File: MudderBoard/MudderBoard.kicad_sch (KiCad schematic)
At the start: 0 parts

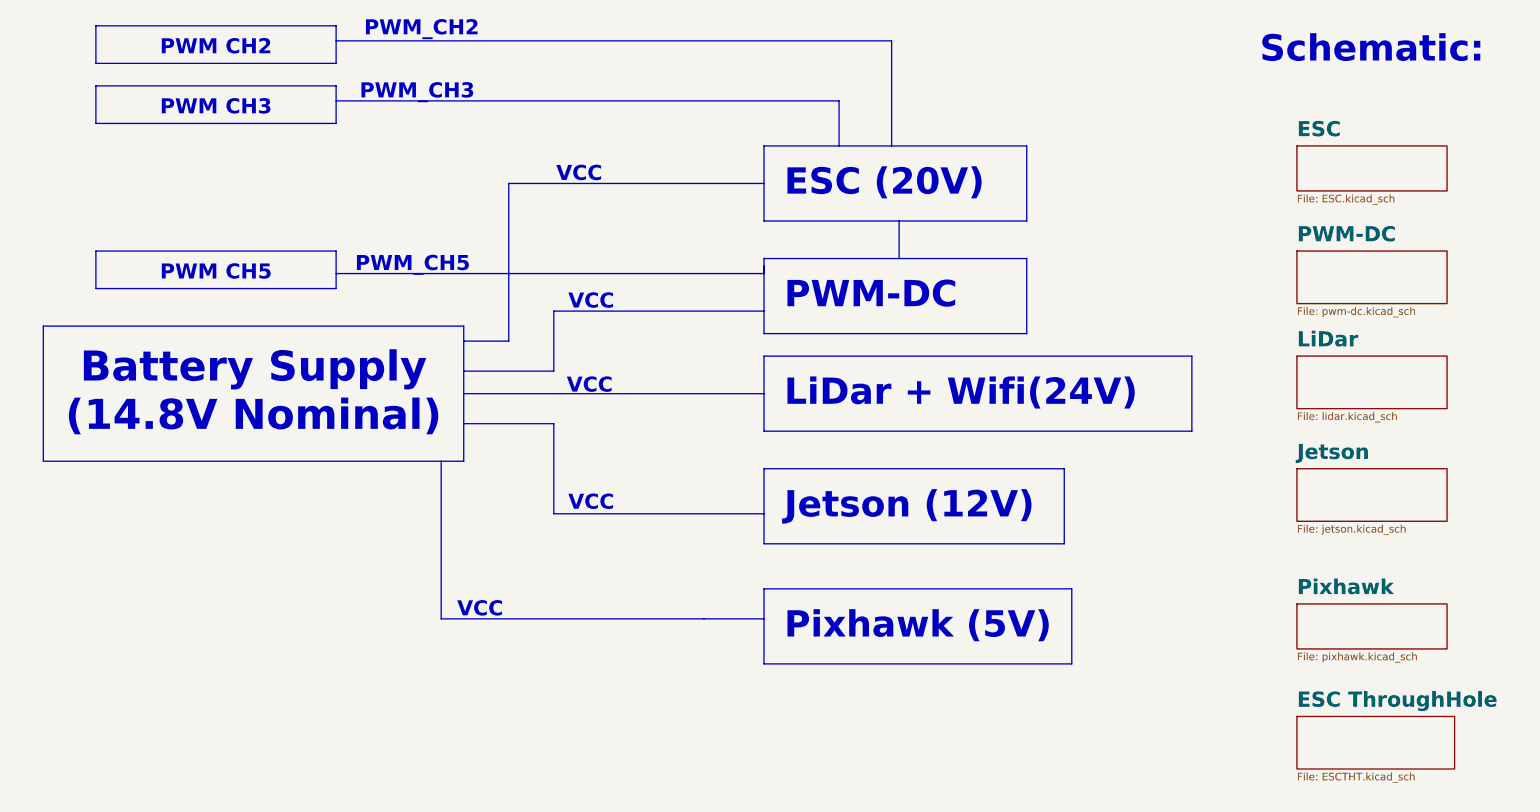
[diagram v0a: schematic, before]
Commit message: added jetson circuit
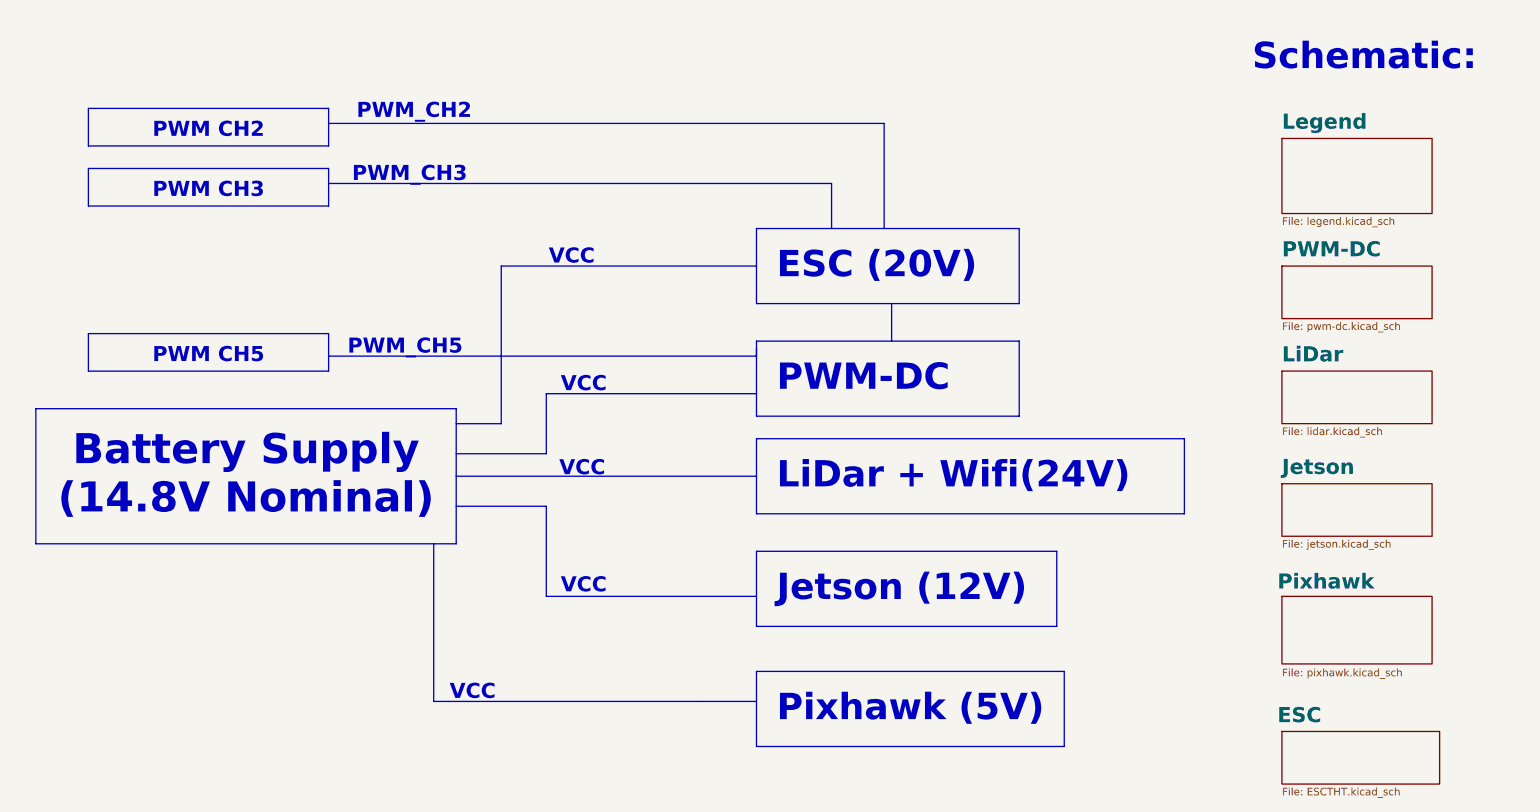
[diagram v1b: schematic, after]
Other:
- removed sheet ESC ThroughHole
- added sheet Legend (legend.kicad_sch)
- sheet ESC: file ESC.kicad_sch -> ESCTHT.kicad_sch
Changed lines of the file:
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@@
 	(polyline
 		(pts
-			(xy 93.98 74.93) (xy 109.22 74.93)
+			(xy 92.71 88.9) (xy 107.95 88.9)
 		)
 		(stroke
@@
 	(polyline
 		(pts
-			(xy 72.39 58.42) (xy 144.78 58.42)
+			(xy 71.12 72.39) (xy 143.51 72.39)
 		)
 		(stroke
@@
 	(polyline
 		(pts
-			(xy 167.64 49.53) (xy 167.64 55.88)
+			(xy 166.37 63.5) (xy 166.37 69.85)
 		)
 		(stroke
@@
 	(polyline
 		(pts
-			(xy 72.39 29.21) (xy 157.48 29.21)
+			(xy 71.12 43.18) (xy 156.21 43.18)
 		)
 		(stroke
@@
 	(polyline
 		(pts
-			(xy 101.6 69.85) (xy 101.6 43.18)
+			(xy 100.33 83.82) (xy 100.33 57.15)
 		)
 		(stroke
@@
 	(polyline
 		(pts
-			(xy 109.22 74.93) (xy 109.22 64.77)
+			(xy 107.95 88.9) (xy 107.95 78.74)
 		)
 		(stroke
@@
 	(polyline
 		(pts
-			(xy 109.22 64.77) (xy 144.78 64.77)
+			(xy 107.95 78.74) (xy 143.51 78.74)
 		)
 		(stroke
@@
 	(polyline
 		(pts
-			(xy 157.48 29.21) (xy 157.48 36.83)
+			(xy 156.21 43.18) (xy 156.21 50.8)
 		)
 		(stroke
@@
 	(polyline
 		(pts
-			(xy 144.78 57.15) (xy 144.78 58.42)
+			(xy 143.51 71.12) (xy 143.51 72.39)
 		)
 		(stroke
@@
 	(polyline
 		(pts
-			(xy 90.17 90.17) (xy 90.17 116.84)
+			(xy 88.9 104.14) (xy 88.9 130.81)
 		)
 		(stroke
@@
 	(polyline
 		(pts
-			(xy 93.98 78.74) (xy 144.78 78.74)
+			(xy 92.71 92.71) (xy 143.51 92.71)
 		)
 		(stroke
@@
 	(polyline
 		(pts
-			(xy 134.62 116.84) (xy 144.78 116.84)
+			(xy 133.35 130.81) (xy 143.51 130.81)
 		)
 		(stroke
@@
 	(polyline
 		(pts
-			(xy 90.17 116.84) (xy 134.62 116.84)
+			(xy 88.9 130.81) (xy 133.35 130.81)
 		)
 		(stroke
@@
 	(polyline
 		(pts
-			(xy 166.37 19.05) (xy 166.37 36.83)
+			(xy 165.1 33.02) (xy 165.1 50.8)
 		)
 		(stroke
@@
 	(polyline
 		(pts
-			(xy 72.39 19.05) (xy 166.37 19.05)
+			(xy 71.12 33.02) (xy 165.1 33.02)
 		)
 		(stroke
@@
 	(polyline
 		(pts
-			(xy 144.78 99.06) (xy 109.22 99.06)
+			(xy 143.51 113.03) (xy 107.95 113.03)
 		)
 		(stroke
@@
 	(polyline
 		(pts
-			(xy 109.22 99.06) (xy 109.22 83.82)
+			(xy 107.95 113.03) (xy 107.95 97.79)
 		)
 		(stroke
@@
 	(polyline
 		(pts
-			(xy 93.98 69.85) (xy 101.6 69.85)
+			(xy 92.71 83.82) (xy 100.33 83.82)
 		)
 		(stroke
@@
 	(polyline
 		(pts
-			(xy 101.6 43.18) (xy 144.78 43.18)
+			(xy 100.33 57.15) (xy 143.51 57.15)
 		)
 		(stroke
@@
 	(polyline
 		(pts
-			(xy 93.98 83.82) (xy 109.22 83.82)
+			(xy 92.71 97.79) (xy 107.95 97.79)
 		)
 		(stroke
@@
 	(text_box "PWM CH2"
 		(exclude_from_sim no)
-		(at 31.75 16.51 0)
+		(at 30.48 30.48 0)
 		(size 40.64 6.35)
 		(stroke
@@
 	(text_box "PWM CH5"
 		(exclude_from_sim no)
-		(at 31.75 54.61 0)
+		(at 30.48 68.58 0)
 		(size 40.64 6.35)
 		(stroke
@@
 	(text_box "Pixhawk (5V)"
 		(exclude_from_sim no)
-		(at 144.78 111.76 0)
+		(at 143.51 125.73 0)
 		(size 52.07 12.7)
 		(stroke
@@
 	(text_box "Jetson (12V)"
 		(exclude_from_sim no)
-		(at 144.78 91.44 0)
+		(at 143.51 105.41 0)
 		(size 50.8 12.7)
 		(stroke
@@
 	(text_box "LiDar + Wifi(24V)"
 		(exclude_from_sim no)
-		(at 144.78 72.39 0)
+		(at 143.51 86.36 0)
 		(size 72.39 12.7)
 		(stroke
@@
 	(text_box "PWM-DC"
 		(exclude_from_sim no)
-		(at 144.78 55.88 0)
+		(at 143.51 69.85 0)
 		(size 44.45 12.7)
 		(stroke
@@
 	(text_box "ESC (20V)"
 		(exclude_from_sim no)
-		(at 144.78 36.83 0)
+		(at 143.51 50.8 0)
 		(size 44.45 12.7)
 		(stroke
@@
 	(text_box "Battery Supply (14.8V Nominal)"
 		(exclude_from_sim no)
-		(at 22.86 67.31 0)
+		(at 21.59 81.28 0)
 		(size 71.12 22.86)
 		(stroke
@@
 	(text_box "PWM CH3"
 		(exclude_from_sim no)
-		(at 31.75 26.67 0)
+		(at 30.48 40.64 0)
 		(size 40.64 6.35)
 		(stroke
@@
 	(text "VCC"
 		(exclude_from_sim no)
-		(at 115.57 63.246 0)
+		(at 114.3 77.216 0)
 		(effects
 			(font
@@
 	(text "PWM_CH3"
 		(exclude_from_sim no)
-		(at 86.106 27.686 0)
+		(at 84.836 41.656 0)
 		(effects
 			(font
@@
 	(text "VCC"
 		(exclude_from_sim no)
-		(at 115.316 77.47 0)
+		(at 114.046 91.44 0)
 		(effects
 			(font
@@
 	(text "PWM_CH2"
 		(exclude_from_sim no)
-		(at 86.868 17.018 0)
+		(at 85.598 30.988 0)
 		(effects
 			(font
@@
 	(text "PWM_CH5"
 		(exclude_from_sim no)
-		(at 85.344 56.896 0)
+		(at 84.074 70.866 0)
 		(effects
 			(font
@@
 	(text "VCC"
 		(exclude_from_sim no)
-		(at 115.57 97.282 0)
+		(at 114.3 111.252 0)
 		(effects
 			(font
@@
 	(text "Schematic:"
 		(exclude_from_sim no)
-		(at 247.65 20.574 0)
+		(at 246.38 21.844 0)
 		(effects
 			(font
@@
 	(text "VCC"
 		(exclude_from_sim no)
-		(at 113.538 41.656 0)
+		(at 112.268 55.626 0)
 		(effects
 			(font
@@
 	(text "VCC"
 		(exclude_from_sim no)
-		(at 96.774 115.316 0)
+		(at 95.504 129.286 0)
 		(effects
 			(font
@@
 	)
 	(sheet
-		(at 234.95 114.3)
-		(size 25.4 7.62)
-		(fields_autoplaced yes)
+		(at 232.41 113.03)
+		(size 25.4 11.43)
 		(stroke
 			(width 0.1524)
@@
 		)
 		(property "Sheetname" "Pixhawk"
-			(at 234.95 112.9534 0)
+			(at 231.648 112.014 0)
 			(effects
 				(font
@@
 		)
 		(property "Sheetfile" "pixhawk.kicad_sch"
-			(at 234.95 122.5046 0)
+			(at 232.41 125.222 0)
 			(effects
 				(font
@@
 	)
 	(sheet
-		(at 234.95 133.35)
+		(at 232.41 135.89)
 		(size 26.67 8.89)
-		(fields_autoplaced yes)
 		(stroke
 			(width 0.1524)
@@
 			(color 0 0 0 0.0000)
 		)
-		(property "Sheetname" "ESC ThroughHole"
-			(at 234.95 132.0034 0)
+		(property "Sheetname" "ESC"
+			(at 231.648 134.62 0)
 			(effects
 				(font
@@
 		)
 		(property "Sheetfile" "ESCTHT.kicad_sch"
-			(at 234.95 142.8246 0)
+			(at 232.41 145.3646 0)
 			(effects
 				(font
@@
 	)
 	(sheet
-		(at 234.95 54.61)
+		(at 232.41 57.15)
 		(size 25.4 8.89)
 		(fields_autoplaced yes)
@@
 		)
 		(property "Sheetname" "PWM-DC"
-			(at 234.95 53.2634 0)
+			(at 232.41 55.8034 0)
 			(effects
 				(font
@@
 		)
 		(property "Sheetfile" "pwm-dc.kicad_sch"
-			(at 234.95 64.0846 0)
+			(at 232.41 66.6246 0)
 			(effects
 				(font
@@
 	)
 	(sheet
-		(at 234.95 36.83)
-		(size 25.4 7.62)
+		(at 232.41 93.98)
+		(size 25.4 8.89)
 		(fields_autoplaced yes)
 		(stroke
@@
 			(color 0 0 0 0.0000)
 		)
-		(property "Sheetname" "ESC"
-			(at 234.95 35.4834 0)
+		(property "Sheetname" "Jetson"
+			(at 232.41 92.6334 0)
 			(effects
 				(font
@@
 			)
 		)
-		(property "Sheetfile" "ESC.kicad_sch"
-			(at 234.95 45.0346 0)
+		(property "Sheetfile" "jetson.kicad_sch"
+			(at 232.41 103.4546 0)
 			(effects
 				(font
@@
 			(project "MudderBoard"
 				(path "/cdf98bf7-80ce-4b13-b655-e6c7c589c122"
-					(page "3")
+					(page "5")
 				)
 			)
@@
 	)
 	(sheet
-		(at 234.95 91.44)
-		(size 25.4 8.89)
+		(at 232.41 35.56)
+		(size 25.4 12.7)
 		(fields_autoplaced yes)
 		(stroke
@@
 			(color 0 0 0 0.0000)
 		)
-		(property "Sheetname" "Jetson"
-			(at 234.95 90.0934 0)
+		(property "Sheetname" "Legend"
+			(at 232.41 34.2134 0)
 			(effects
 				(font
@@
 			)
 		)
-		(property "Sheetfile" "jetson.kicad_sch"
-			(at 234.95 100.9146 0)
+		(property "Sheetfile" "legend.kicad_sch"
+			(at 232.41 48.8446 0)
 			(effects
 				(font
@@
 			(project "MudderBoard"
 				(path "/cdf98bf7-80ce-4b13-b655-e6c7c589c122"
-					(page "5")
+					(page "7")
 				)
 			)
@@
 	)
 	(sheet
-		(at 234.95 72.39)
+		(at 232.41 74.93)
 		(size 25.4 8.89)
 		(fields_autoplaced yes)
@@
 		)
 		(property "Sheetname" "LiDar"
-			(at 234.95 71.0434 0)
+			(at 232.41 73.5834 0)
 			(effects
 				(font
@@
 		)
 		(property "Sheetfile" "lidar.kicad_sch"
-			(at 234.95 81.8646 0)
+			(at 232.41 84.4046 0)
 			(effects
 				(font
